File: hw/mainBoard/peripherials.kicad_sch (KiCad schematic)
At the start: 12 parts, among them J4 Per_Conn1, J4 Per_Conn2, U5 SRDA3.3-4DR2G

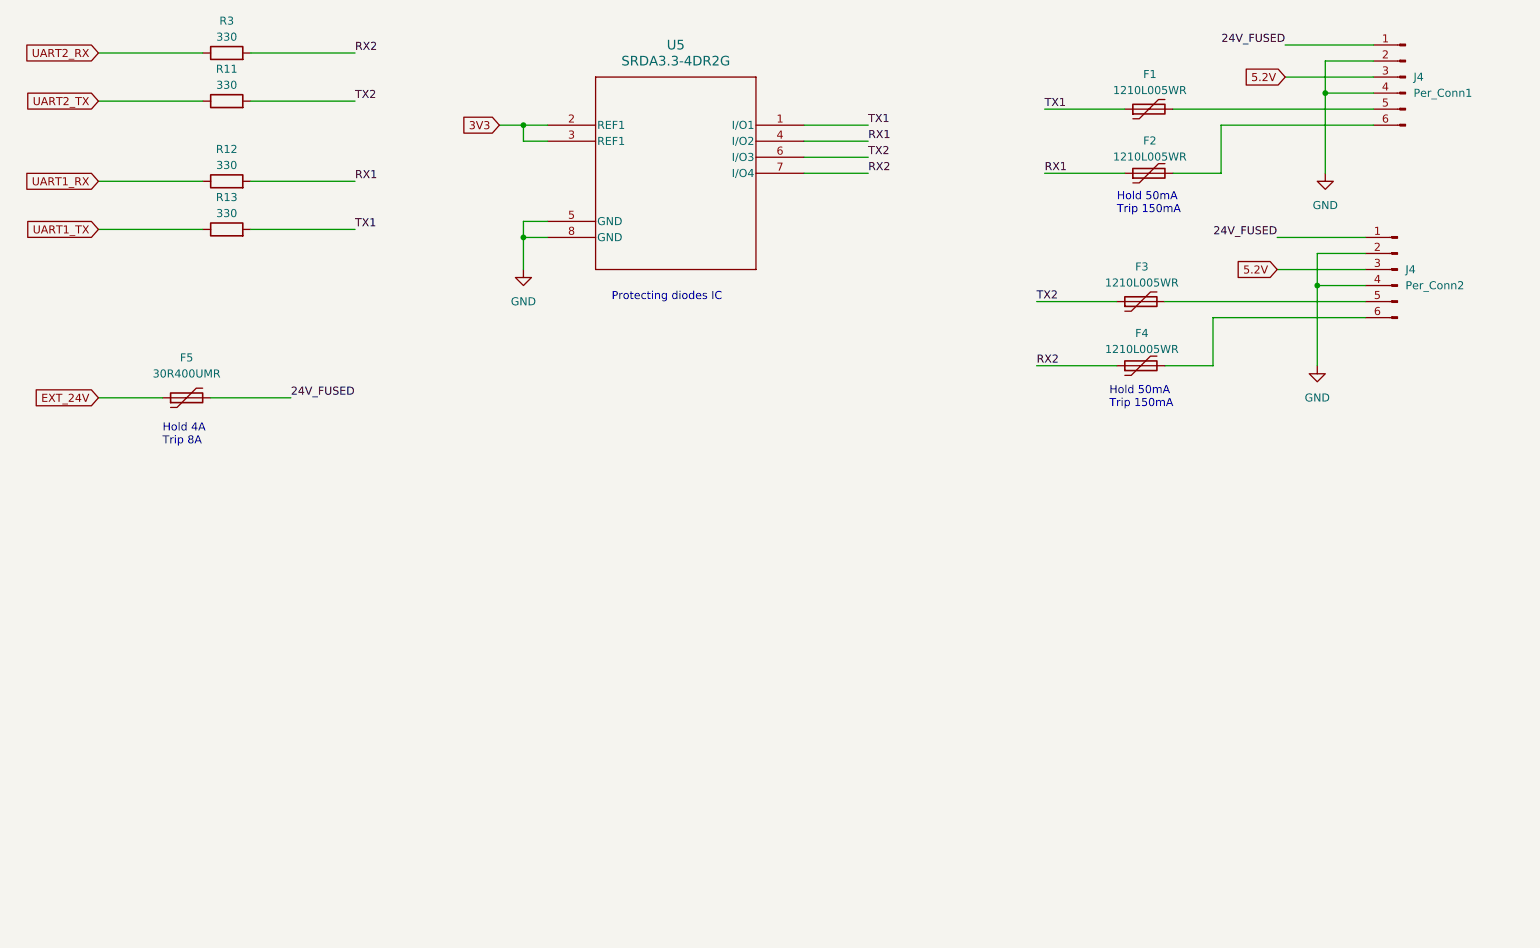
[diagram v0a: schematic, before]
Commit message: hw + blok schema
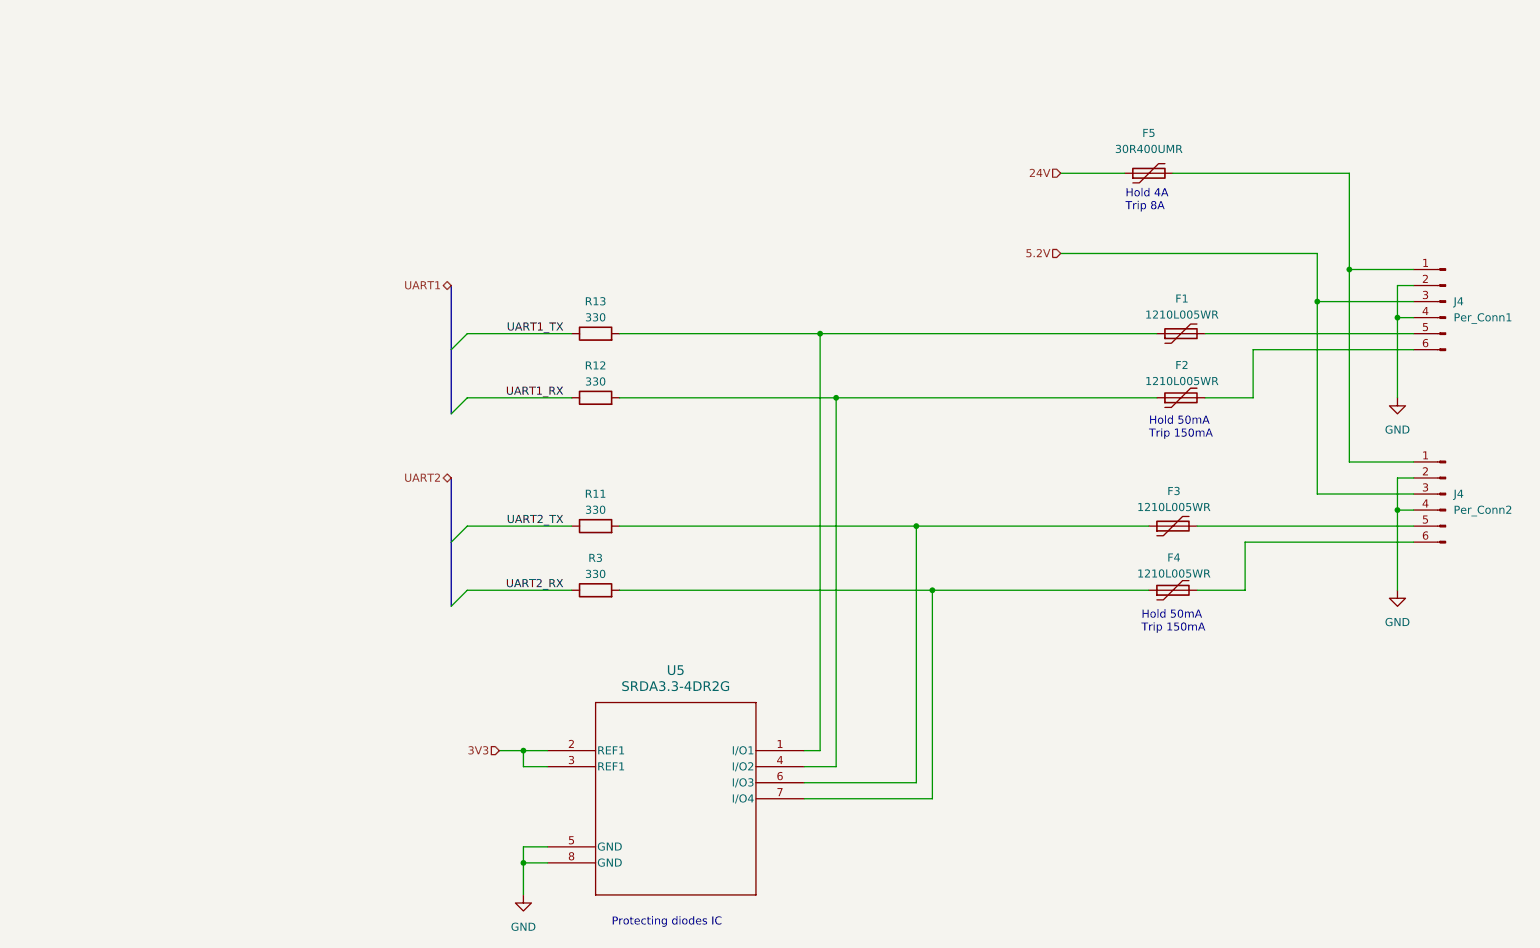
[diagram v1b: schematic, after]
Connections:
- net 24V_FUSED: no longer names the net of F5.2, J4.1 (Pin_1), J4.1 (Pin_1)
- net EXT_24V renamed 24V
- net RX1: no longer names the net of F2.1, R12.2, U5.4 (I/O2)
- net RX2: no longer names the net of F4.1, R3.2, U5.7 (I/O4)
- net TX1: no longer names the net of F1.1, R13.2, U5.1 (I/O1)
- net TX2: no longer names the net of F3.1, R11.2, U5.6 (I/O3)
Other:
- moved on the sheet: F1, F2, F3, F4, F5, J4, R11, R12, R13, R3, U5
